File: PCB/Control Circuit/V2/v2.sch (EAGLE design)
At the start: 6 parts, among them K1 RELAY-SPDT, Q1 60V/32A/35mΩ

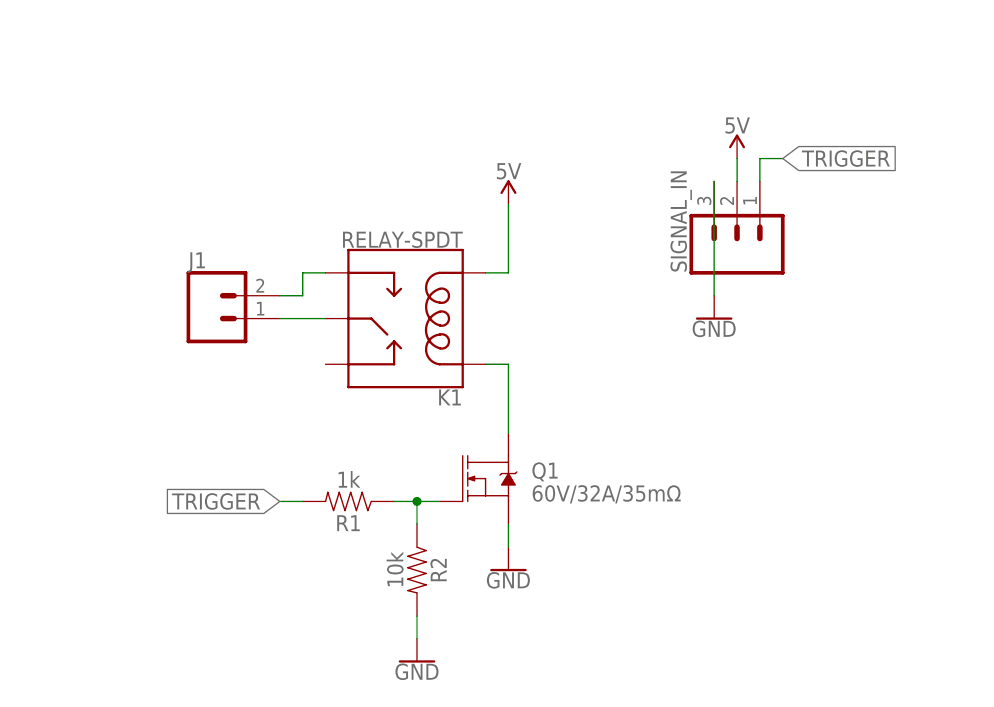
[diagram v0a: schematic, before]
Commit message: Control Circuit v2
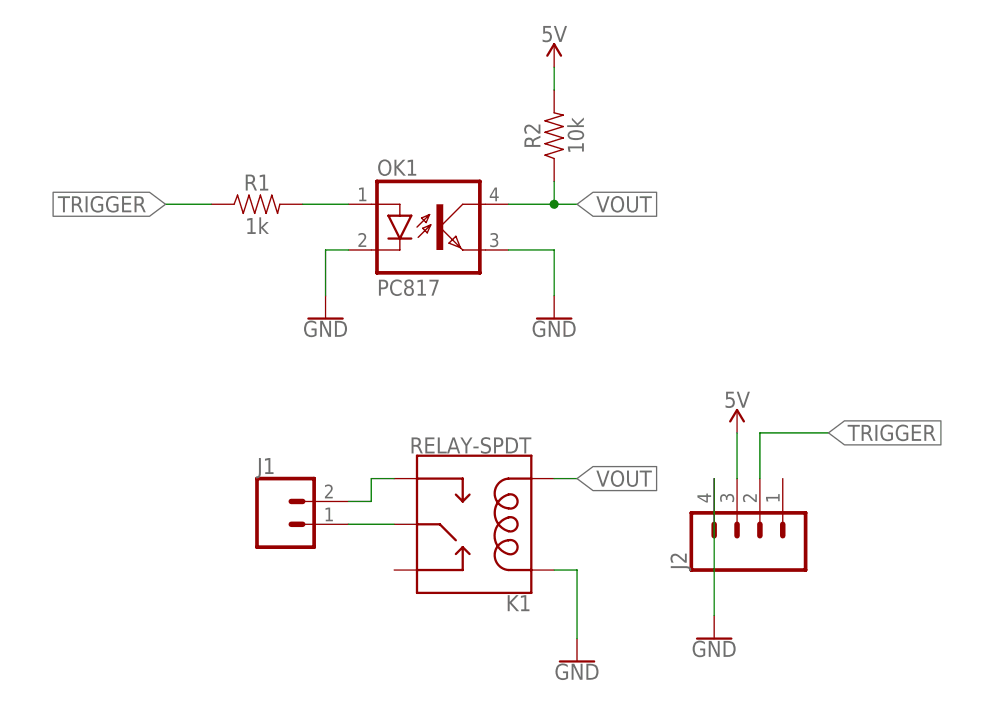
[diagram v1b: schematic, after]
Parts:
- removed Q1: 60V/32A/35mΩ, SparkFun-DiscreteSemi:MOSFET-NCH-FQP30N06L
- removed SIGNAL_IN: (no value), SparkFun-Connectors:CONN_03
- added J2: (no value), SparkFun-Connectors:CONN_04
- added OK1: PC817, optocoupler:PC817
- R2: device SparkFun-Resistors:1KOHM-HORIZ-1/4W-1% -> SparkFun-Resistors:10KOHM-HORIZ-1/4W-1%
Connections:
- removed net N$2: K1.COIL1, Q1.D
- new net VOUT: K1.COIL2, OK1.COL, R2.1
- net 5V: now also J2.3, R2.2; no longer K1.COIL2, SIGNAL_IN.2
- net GND: now also J2.4, K1.COIL1, OK1.C, OK1.EMIT; no longer Q1.S, R2.2, SIGNAL_IN.3
- net N$1: now also OK1.A, R1.2; no longer Q1.G, R1.1, R2.1
- net TRIGGER: now also J2.2, R1.1; no longer R1.2, SIGNAL_IN.1
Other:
- moved on the sheet: J1, K1, R1, R2
